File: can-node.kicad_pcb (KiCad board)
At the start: 2 copper layers, 60 x 60 mm, 54 parts, among them P1 SWD, P2 DEBUG_UART, P3 CONN_01X06, Q1 DMP6023LSS, SW1 SW_PUSH, SW2 SW_PUSH, SW3 SW_PUSH, U1 LMR16006, U2 SN74LVC1G08, U3 STM32F072RB, U4 HDC1080, U5 TCAN334, X1 32.768KHz 12.5pF

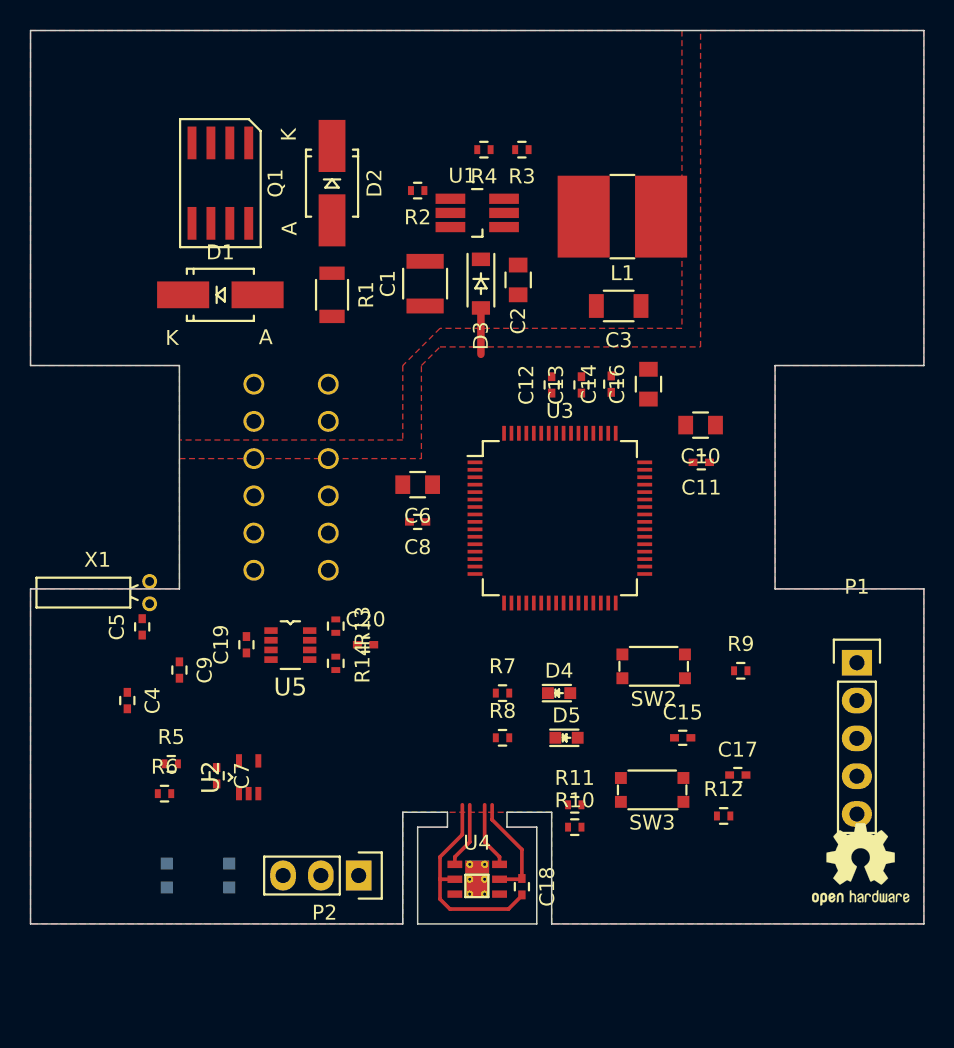
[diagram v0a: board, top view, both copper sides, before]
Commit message: Layout: first version
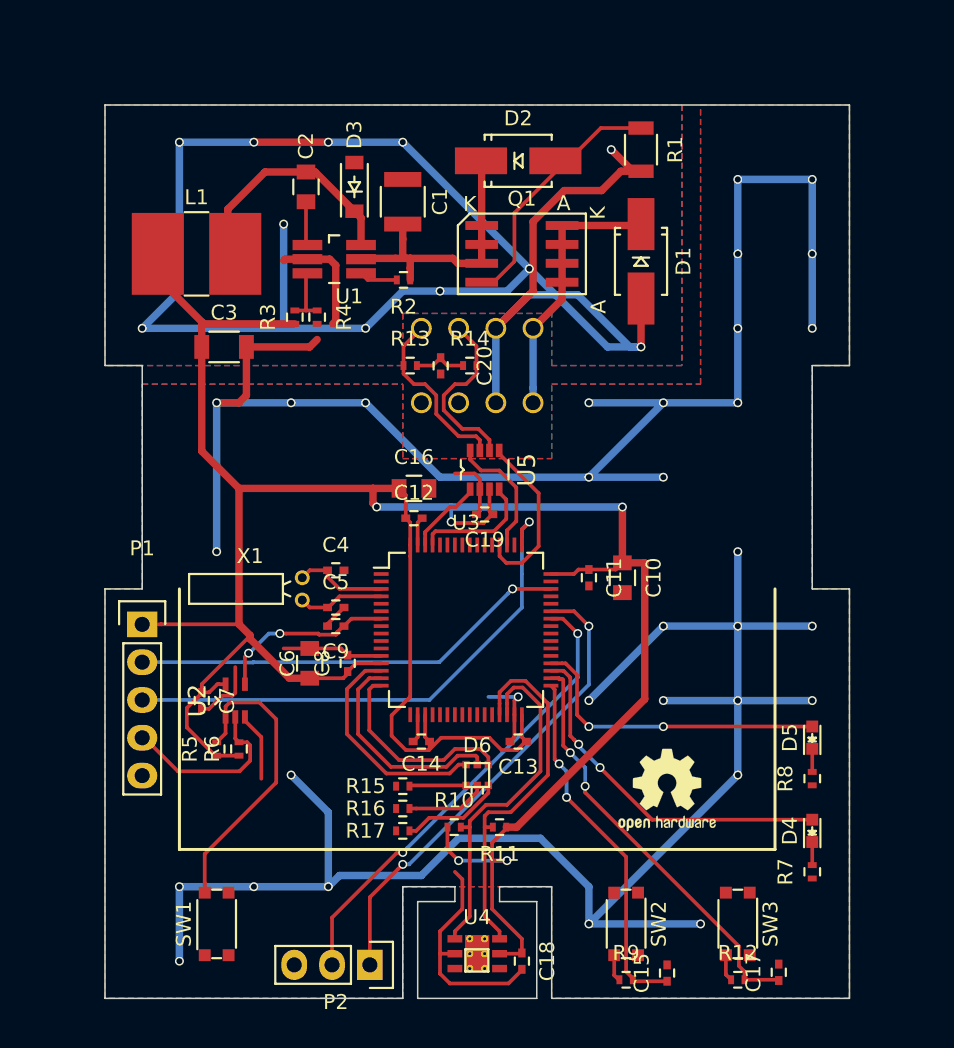
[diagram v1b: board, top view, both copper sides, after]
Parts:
- added D6: LED_RGB_EP, CAN_Node:Everlight_19-337, F.Cu at (145.0, 110.0)
- added R15: 220, Resistors_SMD:R_0402, F.Cu at (140.0, 110.8)
- added R16: 220, Resistors_SMD:R_0402, F.Cu at (140.0, 112.2)
- added R17: 220, Resistors_SMD:R_0402, F.Cu at (140.0, 113.8)
- P3: value CONN_01X06 -> CONN_01X04; footprint CAN_Node:WAGO_218-106 -> CAN_Node:WAGO_218-104
- SW1: moved to F.Cu
- moved P1 48.1 mm to (122.5, 99.9)
- moved L1 28.7 mm to (126.2, 75.0), turned to 180 degrees
- moved D1 28.3 mm to (156.0, 75.5), turned to 270 degrees
- moved C14 27.2 mm to (141.2, 107.8), turned to 180 degrees
- moved C3 26.6 mm to (128.0, 81.2), turned to 0 degrees
- moved C13 24.3 mm to (147.8, 107.8), turned to 180 degrees
- moved R7 24.0 mm to (167.5, 116.5), turned to 90 degrees
- moved R1 22.9 mm to (156.0, 68.0)
- moved R9 22.1 mm to (155.0, 123.8)
- moved R14 21.9 mm to (144.5, 82.5), turned to 0 degrees
- moved R8 21.0 mm to (167.5, 110.2), turned to 90 degrees
- moved Q1 20.8 mm to (148.0, 75.0), turned to 270 degrees
- moved C20 19.4 mm to (142.5, 82.5), turned to 270 degrees
- moved D4 19.4 mm to (167.5, 113.8), turned to 90 degrees
- moved R3 19.0 mm to (132.8, 79.2), turned to 90 degrees
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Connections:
- net Net-(U3-Pad10) renamed /Microcontroller/PC2
- net Net-(U3-Pad11) renamed /Microcontroller/PC3
- net Net-(U3-Pad24) renamed /Microcontroller/PC4
- net Net-(U3-Pad25) renamed /Microcontroller/PC5
- net Net-(U3-Pad28) renamed /Microcontroller/PB2
- net Net-(U3-Pad37) renamed /Microcontroller/PC6
- net Net-(U3-Pad38) renamed /Microcontroller/PC7
- net Net-(U3-Pad57) renamed /Microcontroller/PB5
- net Net-(U3-Pad8) renamed /Microcontroller/PC0
- net Net-(U3-Pad9) renamed /Microcontroller/PC1
- C18 pad 1: Net-(C18-Pad1) -> +3.3VADC
- P2 pad 1: GND -> /Microcontroller/UART1_RX
- P2 pad 2: /Microcontroller/UART_RX -> /Microcontroller/UART1_TX
- P2 pad 3: /Microcontroller/UART_TX -> GND
- P3 pad 3: CANH_IN -> CANL_IN
- P3 pad 4: CANL_IN -> CANH_IN
- R10 pad 2: /Microcontroller/I2C1_SDA -> Net-(R10-Pad2)
- R11 pad 2: /Microcontroller/I2C1_SCL -> Net-(R11-Pad2)
- R13 pad 1: Net-(JP1-Pad2) -> CANH_IN
- U3 pad 16: /Microcontroller/UART_TX -> Net-(D6-Pad4)
- U3 pad 17: /Microcontroller/UART_RX -> Net-(U3-Pad17)
- U3 pad 26: Net-(D4-Pad2) -> /Microcontroller/PB0
- U3 pad 27: Net-(D5-Pad2) -> /Microcontroller/PB1
- U3 pad 29: Net-(U3-Pad29) -> Net-(R11-Pad2)
- U3 pad 30: Net-(U3-Pad30) -> Net-(R10-Pad2)
- U3 pad 33: Net-(U3-Pad33) -> Net-(C15-Pad1)
- U3 pad 34: Net-(U3-Pad34) -> Net-(C17-Pad1)
- U3 pad 35: Net-(U3-Pad35) -> Net-(D4-Pad2)
- U3 pad 36: Net-(U3-Pad36) -> Net-(D5-Pad2)
- U3 pad 42: Net-(U3-Pad42) -> /Microcontroller/UART1_TX
- U3 pad 43: Net-(U3-Pad43) -> /Microcontroller/UART1_RX
- U3 pad 51: Net-(U3-Pad51) -> CAN_STANDBY
- U3 pad 52: Net-(C15-Pad1) -> CAN_SHUTDOWN
- U3 pad 53: Net-(C17-Pad1) -> Net-(U3-Pad53)
- U3 pad 55: CAN_SHUTDOWN -> /Microcontroller/PB3
- U3 pad 56: CAN_STANDBY -> /Microcontroller/PB4
- U3 pad 58: /Microcontroller/I2C1_SCL -> /Microcontroller/PB6
- U3 pad 59: /Microcontroller/I2C1_SDA -> /Microcontroller/PB7
- U4 pad 1: /Microcontroller/I2C1_SDA -> Net-(R10-Pad2)
- U4 pad 5: Net-(C18-Pad1) -> +3.3VADC
- U4 pad 6: /Microcontroller/I2C1_SCL -> Net-(R11-Pad2)
- X1 pad 1: Net-(C4-Pad1) -> Net-(C5-Pad1)
- X1 pad 2: Net-(C5-Pad1) -> Net-(C4-Pad1)
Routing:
- net GND: track 17.3 -> 277.8 mm, vias 0 -> 27
- net +3.3VADC: track 0.00 -> 184.9 mm, vias 0 -> 5
- net (no net): track 0.00 -> 109.9 mm, vias 0 -> 16
- net /Microcontroller/SWCLK: track 0.00 -> 35.8 mm, vias 0 -> 1
- net /Microcontroller/UART1_RX: track 0.00 -> 32.1 mm, vias 0 -> 2
- net /Microcontroller/UART1_TX: track 0.00 -> 31.5 mm, vias 0 -> 2
- net /Microcontroller/SWDIO: track 0.00 -> 29.5 mm, vias 0 -> 1
- net Net-(C17-Pad1): track 0.00 -> 28.4 mm, vias 0 -> 2
- net Net-(R11-Pad2): track 0.00 -> 25.1 mm
- net Net-(C15-Pad1): track 0.00 -> 24.4 mm, vias 0 -> 2
- net Net-(D4-Pad2): track 0.00 -> 24.1 mm, vias 0 -> 2
- net Net-(R10-Pad2): track 0.00 -> 23.8 mm
- net Net-(D5-Pad2): track 0.00 -> 20.9 mm, vias 0 -> 2
- net Net-(R5-Pad2): track 0.00 -> 20.3 mm
- net Net-(C1-Pad1): track 0.00 -> 18.9 mm
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- added copper zone on B.Cu, net GND
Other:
- board size 60 x 60 mm -> 50 x 60 mm
